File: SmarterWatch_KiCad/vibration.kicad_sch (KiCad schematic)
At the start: 4 parts, among them M1 Motor_DC, Q4 2N7002

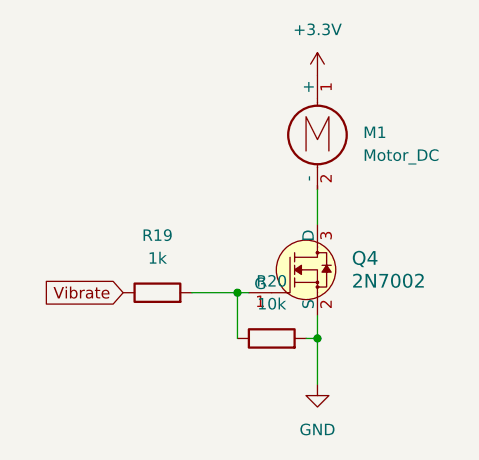
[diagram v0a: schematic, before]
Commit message: Minor Changes
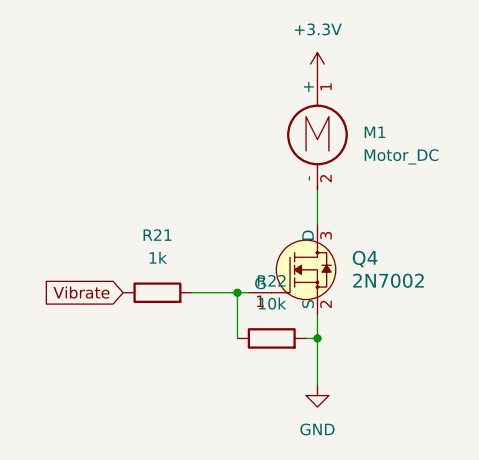
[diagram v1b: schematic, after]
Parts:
- renumbered R19 to R21, R20 to R22
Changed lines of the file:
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@@
 		(dnp no)
 		(fields_autoplaced yes)
-		(property "Reference" "#PWR064"
+		(property "Reference" "#PWR070"
 			(at 74.93 63.5 0)
 			(effects
@@
 			(project "Smarter Watch Stuff"
 				(path "/52181fb0-1be8-41da-83b2-7d5a62778ff4/4391aa75-64c4-4f2b-91f2-dcfd546de819"
-					(reference "#PWR064")
+					(reference "#PWR070")
 					(unit 1)
 				)
@@
 		(dnp no)
 		(fields_autoplaced yes)
-		(property "Reference" "#PWR063"
+		(property "Reference" "#PWR069"
 			(at 74.93 26.67 0)
 			(effects
@@
 			(project "Smarter Watch Stuff"
 				(path "/52181fb0-1be8-41da-83b2-7d5a62778ff4/4391aa75-64c4-4f2b-91f2-dcfd546de819"
-					(reference "#PWR063")
+					(reference "#PWR069")
 					(unit 1)
 				)
@@
 		(dnp no)
 		(fields_autoplaced yes)
-		(property "Reference" "R19"
+		(property "Reference" "R21"
 			(at 57.15 40.64 90)
 			(effects
@@
 			(project "Smarter Watch Stuff"
 				(path "/52181fb0-1be8-41da-83b2-7d5a62778ff4/4391aa75-64c4-4f2b-91f2-dcfd546de819"
-					(reference "R19")
+					(reference "R21")
 					(unit 1)
 				)
@@
 		(dnp no)
 		(fields_autoplaced yes)
-		(property "Reference" "R20"
+		(property "Reference" "R22"
 			(at 69.85 45.72 90)
 			(effects
@@
 			(project "Smarter Watch Stuff"
 				(path "/52181fb0-1be8-41da-83b2-7d5a62778ff4/4391aa75-64c4-4f2b-91f2-dcfd546de819"
-					(reference "R20")
+					(reference "R22")
 					(unit 1)
 				)

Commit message: sync
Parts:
- M1: footprint Smarter watching stuff foot:Vibration motor -> Custom_Foot:Vibration_Motor
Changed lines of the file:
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@@
 			)
 		)
-		(property "Footprint" "Smarter watching stuff foot:Vibration motor"
+		(property "Footprint" "Custom_Foot:Vibration_Motor"
 			(at 74.93 30.226 0)
 			(effects
